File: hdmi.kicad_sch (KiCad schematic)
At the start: 10 parts, among them J8 DC3RX19JA2

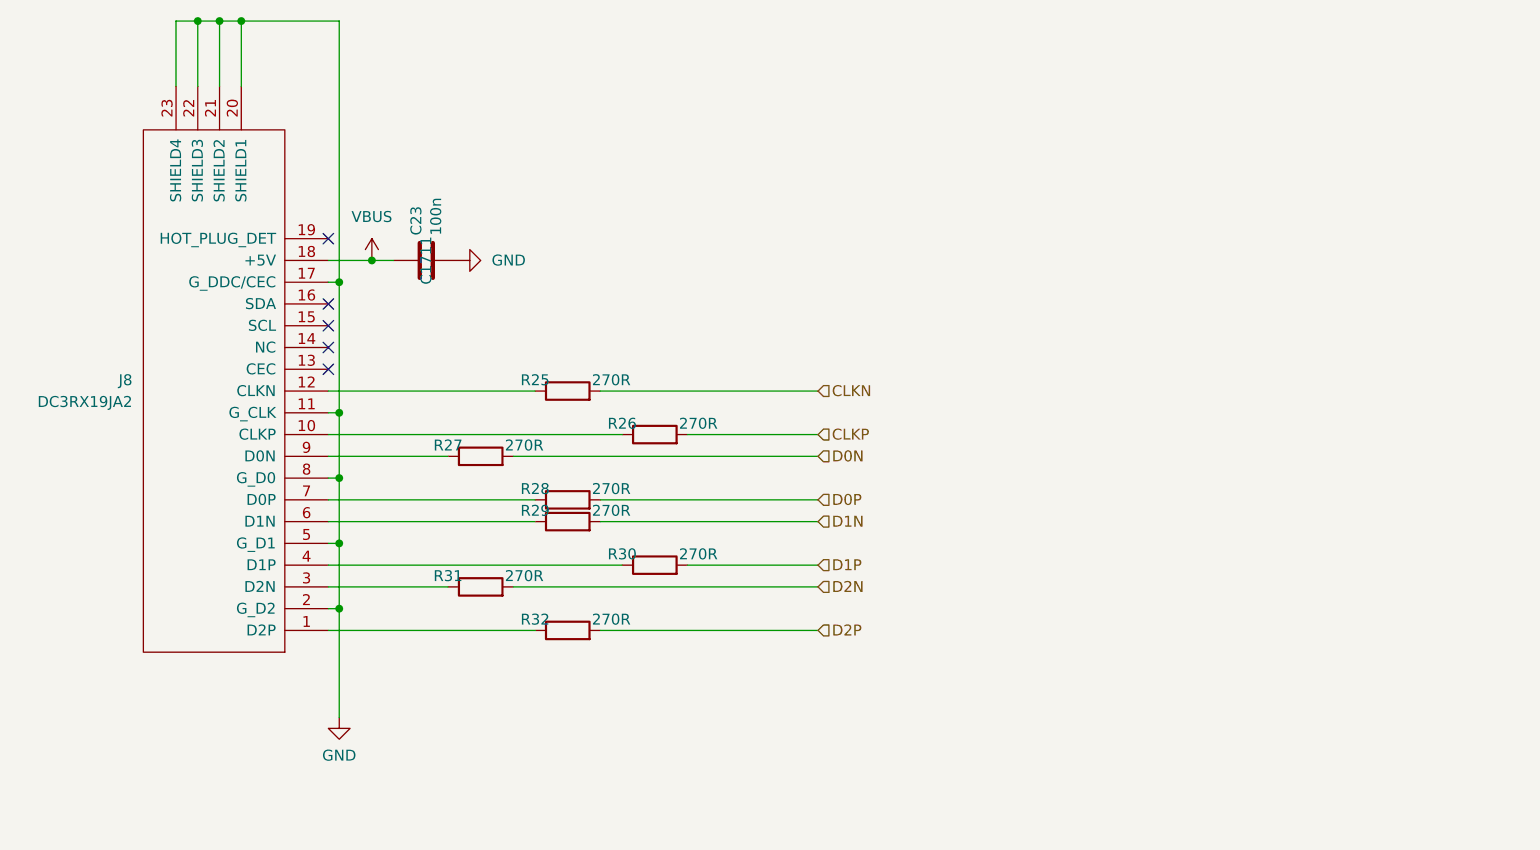
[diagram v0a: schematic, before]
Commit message: Minor fixes
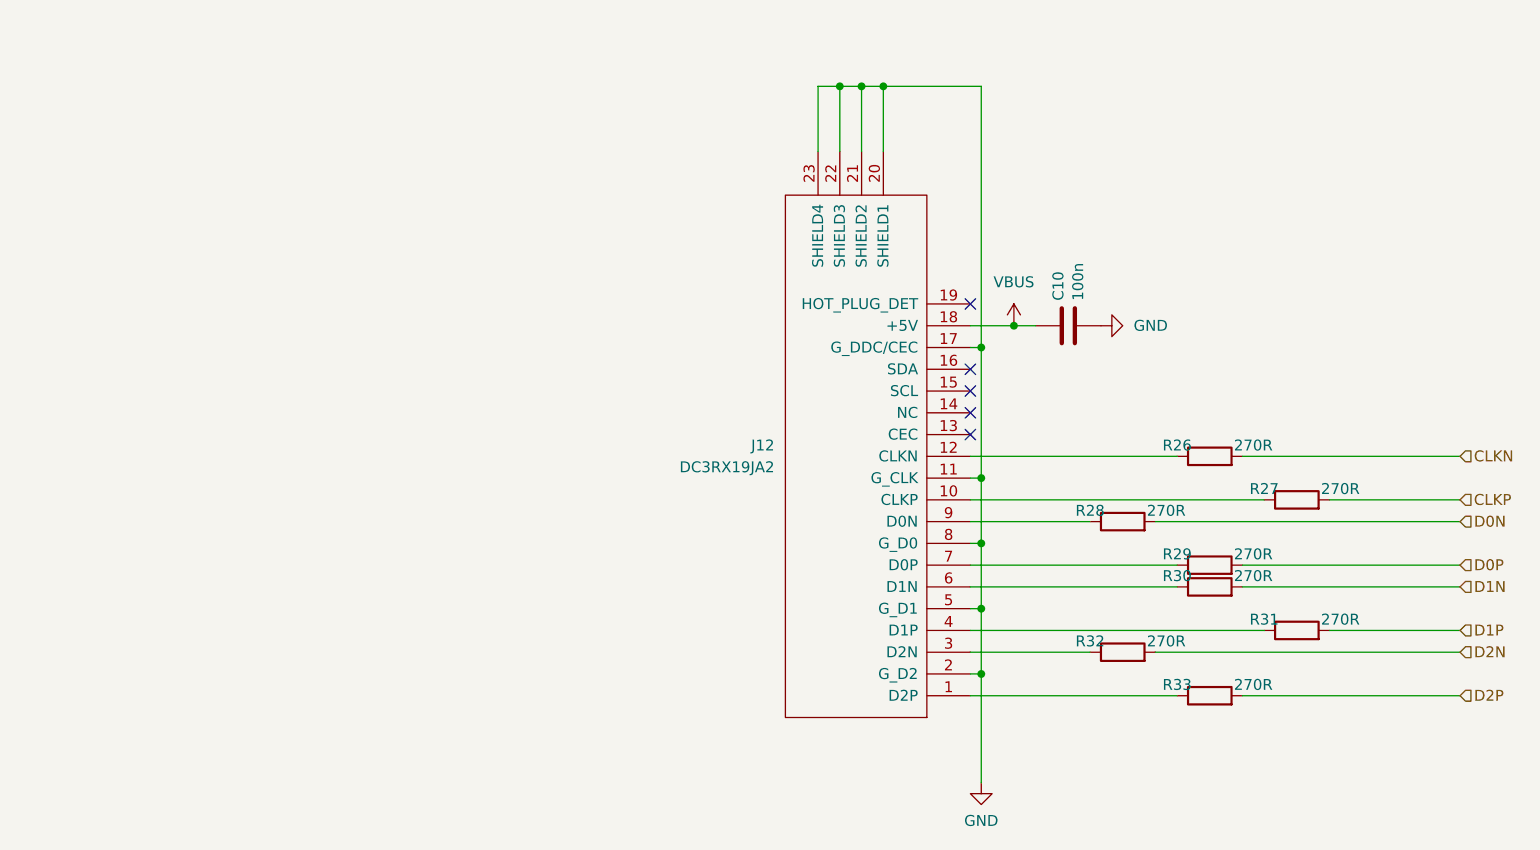
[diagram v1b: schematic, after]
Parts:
- C10: renamed from C23; LCSC C1711 -> (none)
- renumbered J8 to J12, R25 to R26, R26 to R27, R27 to R28, R28 to R29, R29 to R30, R30 to R31, R31 to R32, R32 to R33
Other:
- title: ${NAME} -> MiniFRANK RM1P2
- moved on the sheet: C10, J12, R26, R27, R28, R29, R30, R31, R32, R33
